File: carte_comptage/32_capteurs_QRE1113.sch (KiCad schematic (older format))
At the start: 96 parts, among them U1 QRE1113GR, U10 QRE1113GR, U11 QRE1113GR, U12 QRE1113GR, U13 QRE1113GR, U14 QRE1113GR, U15 QRE1113GR, U16 QRE1113GR, U17 QRE1113GR, U18 QRE1113GR, U19 QRE1113GR, U2 QRE1113GR, U20 QRE1113GR, U21 QRE1113GR, U22 QRE1113GR, U23 QRE1113GR, U24 QRE1113GR, U25 QRE1113GR, U26 QRE1113GR, U27 QRE1113GR, U28 QRE1113GR, U29 QRE1113GR, U3 QRE1113GR, U30 QRE1113GR, U31 QRE1113GR, U32 QRE1113GR, U4 QRE1113GR, U5 QRE1113GR, U6 QRE1113GR, U7 QRE1113GR, U8 QRE1113GR, U9 QRE1113GR

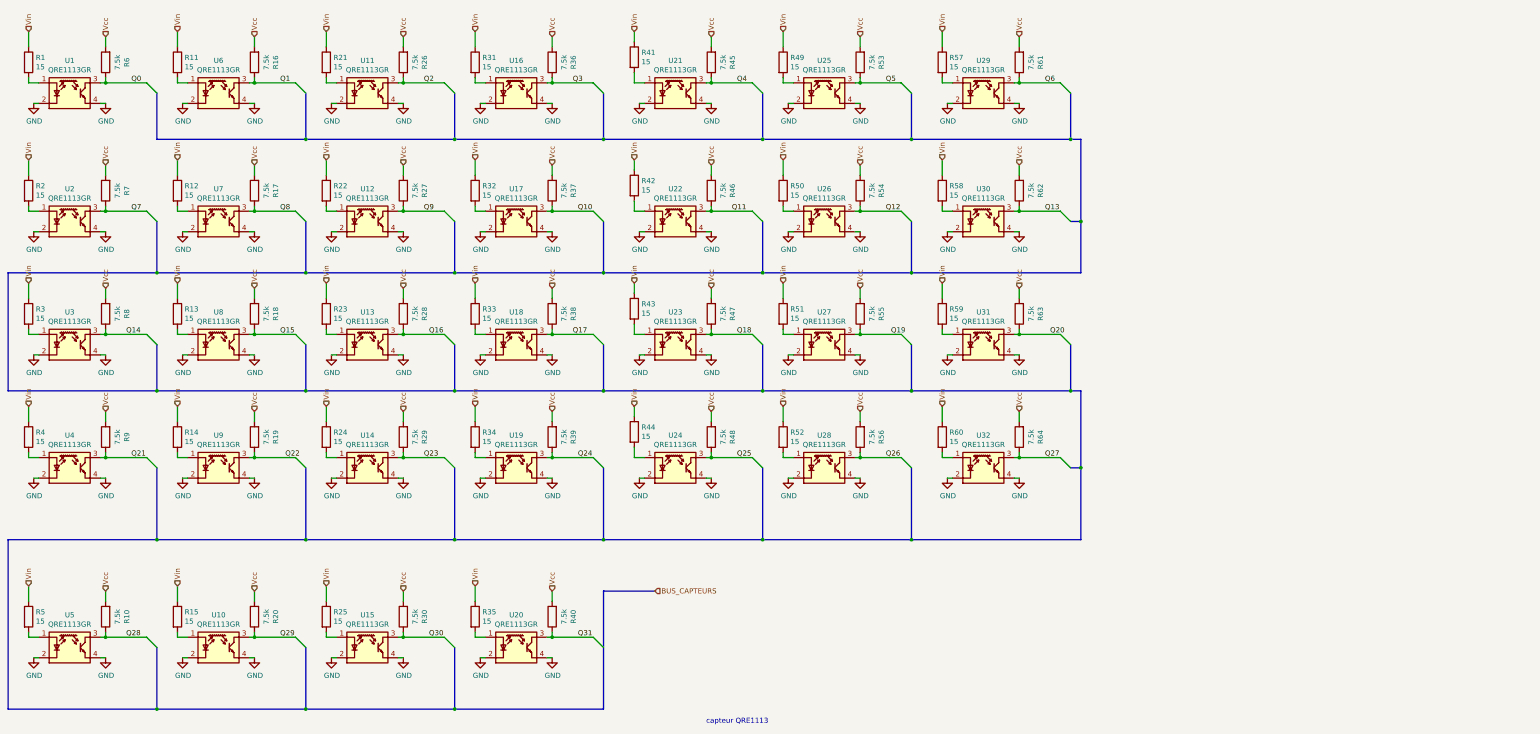
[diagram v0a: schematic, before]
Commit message: DEBUT ROUTAGE
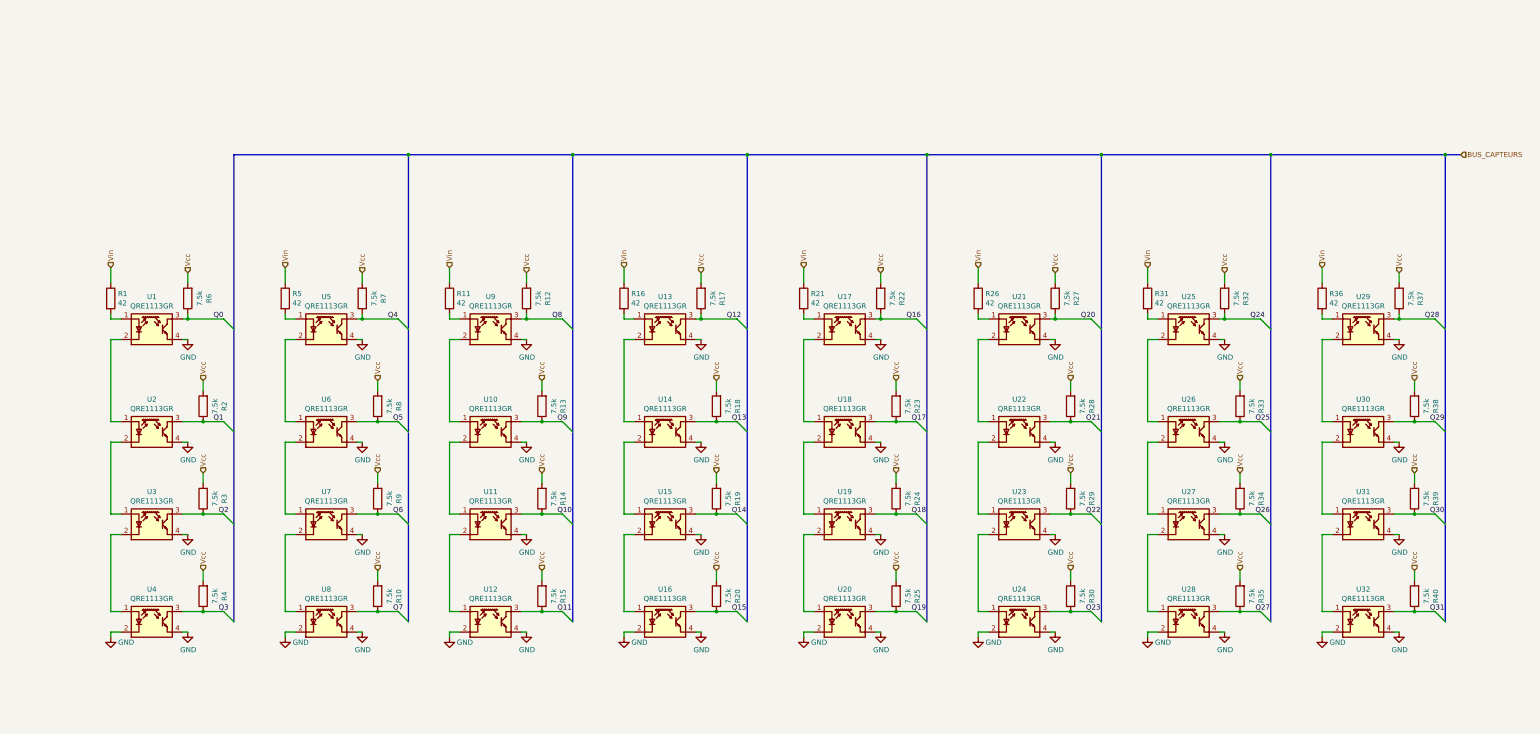
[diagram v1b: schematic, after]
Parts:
- removed R1, R41, R43, R44, R46, R48, R50, R53, R55, R57, R59, R6, R61, R63: 15, Resistor_SMD:R_1206_3216Metric, symbol Device:R
- removed R42, R45, R47, R49, R51, R52, R54, R56, R58, R60, R62, R64: 7.5k, Resistor_SMD:R_1206_3216Metric, symbol Device:R
- added R2, R3: 7.5k, Resistor_SMD:R_1206_3216Metric, symbol Device:R
- R11, R16, R2, R36: value 15 -> 42
- R13, R15, R18, R20, R22, R25, R27, R29, R30, R32, R34, R39, R4, R8: value 15 -> 7.5k
- R21, R26, R31, R5: value 7.5k -> 42
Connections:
- net GND: no longer U1.2 (K), U10.2 (K), U11.2 (K), U13.2 (K), U14.2 (K), U15.2 (K), U17.2 (K), U18.2 (K), U19.2 (K), U2.2 (K), U21.2 (K), U22.2 (K), U23.2 (K), U25.2 (K), U26.2 (K), U27.2 (K), U29.2 (K), U3.2 (K), U30.2 (K), U31.2 (K), U5.2 (K), U6.2 (K), U7.2 (K), U9.2 (K)
- net Q1: now also R2.1; no longer R5.1
- net Q10: now also R14.1; no longer R23.1
- net Q11: now also R15.1; no longer R24.1
- net Q12: now also R17.1; no longer R26.1
- net Q13: now also R18.1; no longer R28.1
- net Q14: now also R19.1; no longer R31.1
- net Q15: now also R20.1; no longer R33.1
- net Q16: now also R22.1; no longer R35.1
- net Q17: now also R23.1; no longer R37.1
- net Q18: now also R24.1; no longer R38.1
- net Q19: now also R25.1; no longer R40.1
- net Q2: now also R3.1; no longer R7.1
- net Q20: now also R27.1
- net Q21: now also R28.1
- net Q22: now also R29.1
- net Q23: now also R30.1
- net Q24: now also R32.1
- net Q25: now also R33.1
- net Q26: now also R34.1
- net Q27: now also R35.1
- net Q28: now also R37.1
- net Q29: now also R38.1
- net Q3: now also R4.1; no longer R9.1
- net Q30: now also R39.1
- net Q31: now also R40.1
- net Q4: now also R7.1; no longer R10.1
- net Q5: now also R8.1; no longer R12.1
- net Q6: now also R9.1; no longer R14.1
- net Q7: now also R10.1; no longer R17.1
- net Q8: now also R12.1; no longer R19.1
- net Q9: now also R13.1; no longer R21.1
- net Vcc: now also R13.2, R15.2, R18.2, R20.2, R22.2, R25.2, R27.2, R29.2, R30.2, R32.2, R34.2, R39.2, R4.2, R8.2, R2.2, R3.2; no longer R21.2, R26.2, R31.2, R5.2
- net Vin: now also R21.1, R26.1, R31.1, R5.1; no longer R13.1, R15.1, R18.1, R20.1, R22.1, R25.1, R27.1, R29.1, R30.1, R32.1, R34.1, R39.1, R4.1, R8.1
- net at U2.1 (A): now also U1.2 (K); no longer R4.2
- net at U3.1 (A): now also U2.2 (K)
- net at U4.1 (A): now also U3.2 (K); no longer R8.2
- net at U5.1 (A): now also R5.2
- net at U6.1 (A): now also U5.2 (K); no longer R11.2
- net at U7.1 (A): now also U6.2 (K); no longer R13.2
- net at U8.1 (A): now also U7.2 (K); no longer R16.2
- net at U9.1 (A): now also R11.2; no longer R18.2
- net at U10.1 (A): now also U9.2 (K); no longer R20.2
- net at U11.1 (A): now also U10.2 (K); no longer R22.2
- net at U12.1 (A): now also U11.2 (K); no longer R15.2
- net at U13.1 (A): now also R16.2; no longer R25.2
- net at U14.1 (A): now also U13.2 (K); no longer R27.2
- net at U15.1 (A): now also U14.2 (K); no longer R30.2
- net at U16.1 (A): now also U15.2 (K); no longer R32.2
- net at U17.1 (A): now also R21.2; no longer R34.2
- net at U18.1 (A): now also U17.2 (K); no longer R36.2
- net at U19.1 (A): now also U18.2 (K); no longer R29.2
- net at U20.1 (A): now also U19.2 (K); no longer R39.2
- net at U21.1 (A): now also R26.2
- net at U22.1 (A): now also U21.2 (K)
- net at U23.1 (A): now also U22.2 (K)
- net at U24.1 (A): now also U23.2 (K)
- net at U25.1 (A): now also R31.2
- net at U26.1 (A): now also U25.2 (K)
- net at U27.1 (A): now also U26.2 (K)
- net at U28.1 (A): now also U27.2 (K)
- net at U29.1 (A): now also R36.2
- net at U30.1 (A): now also U29.2 (K)
- net at U31.1 (A): now also U30.2 (K)
- net at U32.1 (A): now also U31.2 (K)
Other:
- note removed: "capteur QRE1113\n"
- moved on the sheet: R1, R6, U1
